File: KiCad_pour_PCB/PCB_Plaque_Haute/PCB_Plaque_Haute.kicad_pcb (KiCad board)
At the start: 2 copper layers, 108 x 108 mm, 9 parts

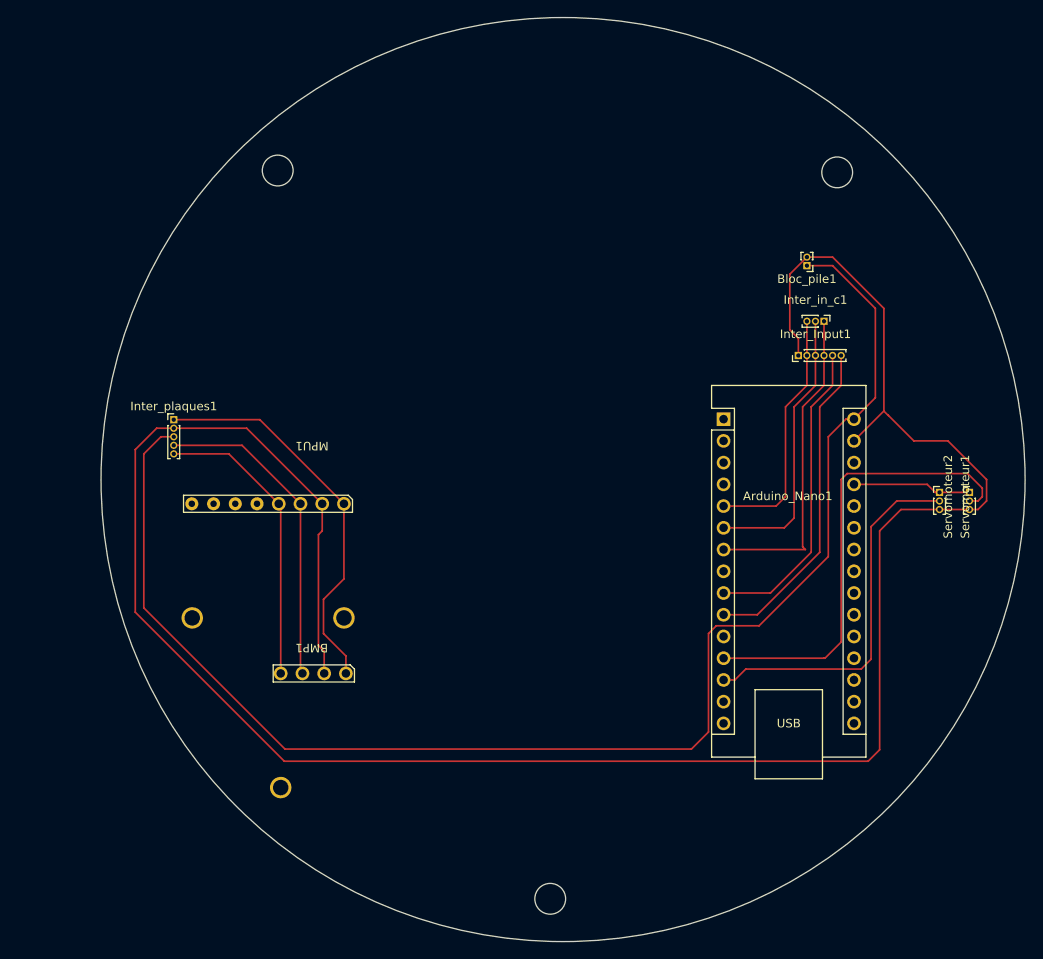
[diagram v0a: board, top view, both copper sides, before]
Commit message: Avancement carte PCB
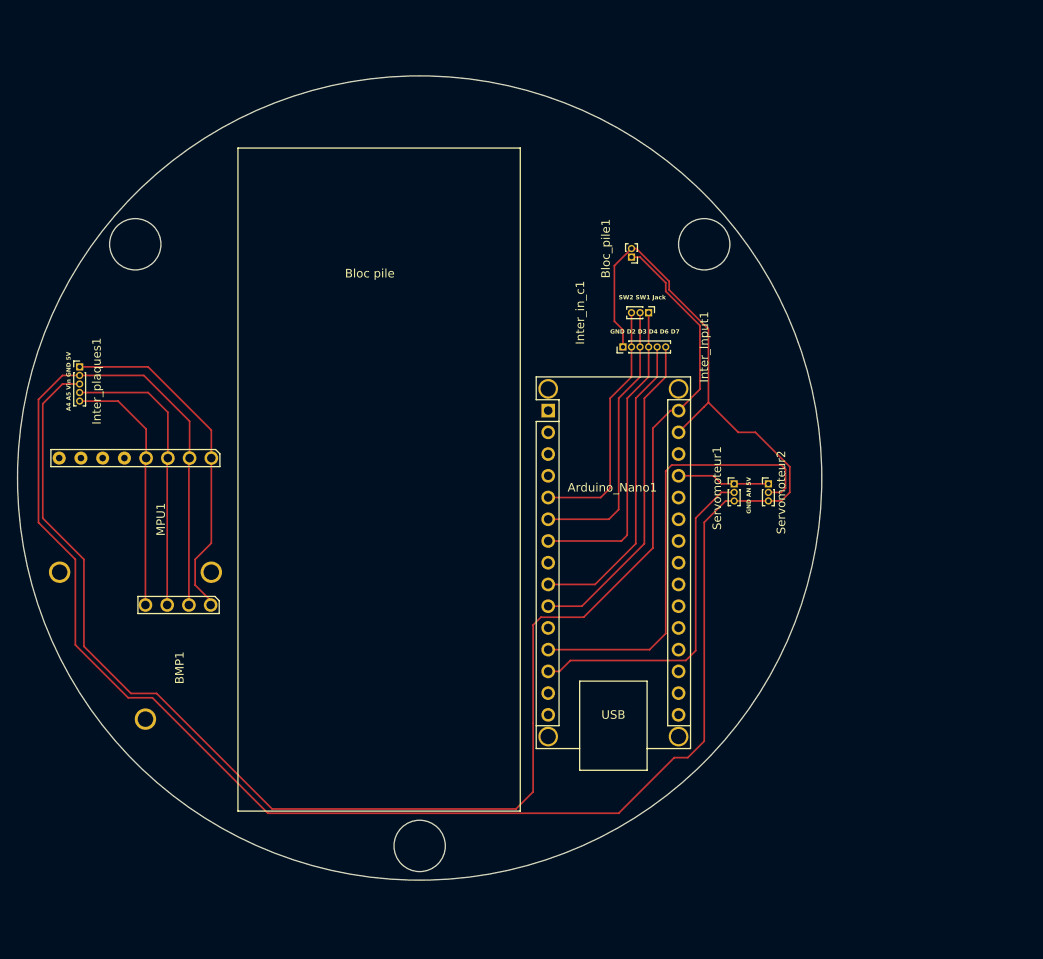
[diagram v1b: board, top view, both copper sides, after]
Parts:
- moved Servomoteur1 24.0 mm to (192.5, 100.0)
- moved Servomoteur2 23.5 mm to (196.5, 100.0)
- moved Arduino_Nano1 20.5 mm to (170.8, 91.4)
- moved Bloc_pile1 20.5 mm to (180.5, 73.5)
- moved Inter_Input1 20.5 mm to (179.5, 84.0)
- moved Inter_in_c1 20.5 mm to (182.5, 80.0)
- moved BMP1 17.7 mm to (131.3, 114.2)
- moved MPU1 16.4 mm to (131.4, 97.0)
- moved Inter_plaques1 12.6 mm to (116.0, 86.3)
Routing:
- net Net-(BMP1-GND): track 259.1 -> 250.5 mm
- net Net-(Arduino_Nano1-Vin): track 167.1 -> 174.8 mm
- net Net-(BMP1-VCC): track 45.9 -> 40.4 mm
- net Net-(BMP1-SDA): track 34.6 -> 29.7 mm
- net Net-(BMP1-SCL): track 37.6 -> 33.8 mm
- net Net-(Arduino_Nano1-D10): track 43.0 -> 39.5 mm
- net Net-(Arduino_Nano1-5V): track 13.9 -> 10.9 mm
- net Net-(Arduino_Nano1-D9): track 53.7 -> 52.4 mm
- net Net-(Arduino_Nano1-D4): track 37.4 -> 36.6 mm
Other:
- board size 108 x 108 mm -> 94 x 94 mm
- board text added: "A4 A5 Vin GND 5V"
- board text added: "GND AN 5V"
- board text added: "GND D2 D3 D4 D6 D7"
- board text added: "SW2 SW1 Jack"
